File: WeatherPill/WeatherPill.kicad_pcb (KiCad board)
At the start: 2 copper layers, 319.5 x 201 mm, 61 parts, among them J1 Conn_01x02_Pin, J2 12402012E212A, J3 Conn_02x04_Odd_Even, J4 Conn_02x05_Odd_Even, J5 Conn_02x08_Odd_Even, Q1 PMOS, Q2 PMOS, SW2 SW_DPDT_x2, SW3 EVQ-P7A01P, SW4 EVQ-P7A01P, U1 USBLC6-2SC6, U2 STM32L052K8Tx, U3 sst25vf512a-33-4c-sae, U4 BU9796AMUV-E2, U5 BME280

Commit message: fred: avancements
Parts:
- removed the R1 at (26.6, 53.5)
- removed the R1 at (20.9, 67.5)
- removed the R15 at (108.5, 65.5)
- removed the R15 at (86.5, 94.5)
- removed R4: 0R, Capacitor_SMD:C_0603_1608Metric_Pad1.08x0.95mm_HandSolder
- added D1: LTST-C190GKT, green led:LEDM1608X80, F.Cu at (29.5, 70.0)
- added D2: LTST-C190GKT, green led:LEDM1608X80, F.Cu at (57.2, 65.5)
- added D3: LTST-C190GKT, green led:LEDM1608X80, F.Cu at (56.8, 86.0)
- added R1: 0R, Capacitor_SMD:C_0603_1608Metric_Pad1.08x0.95mm_HandSolder, F.Cu at (31.4, 47.5)
- added R15: 0R, Capacitor_SMD:C_0603_1608Metric_Pad1.08x0.95mm_HandSolder, F.Cu at (100.0, 45.0)
- added R29: 240R, Resistor_SMD:R_0603_1608Metric_Pad0.98x0.95mm_HandSolder, F.Cu at (31.0, 69.0)
- added R30: 240R, Resistor_SMD:R_0603_1608Metric_Pad0.98x0.95mm_HandSolder, F.Cu at (54.7, 66.0)
- added R31: 240R, Resistor_SMD:R_0603_1608Metric_Pad0.98x0.95mm_HandSolder, F.Cu at (54.3, 86.5)
- BT1: moved to B.Cu
- moved H1 63.8 mm to (107.0, 67.0)
- moved H2 63.8 mm to (107.5, 79.5)
- moved H3 63.8 mm to (89.5, 80.5)
- moved H4 63.8 mm to (103.5, 91.5)
- moved SW4 49.8 mm to (29.5, 88.7), turned to 0 degrees
- moved SW3 49.6 mm to (37.5, 88.7), turned to 0 degrees
- moved R21 48.4 mm to (95.1, 46.5), turned to 0 degrees
- moved R22 45.6 mm to (95.1, 49.0), turned to 0 degrees
- moved R28 45.0 mm to (89.0, 53.0), turned to 0 degrees
- moved R8 43.8 mm to (41.7, 86.2), turned to 0 degrees
- moved C6 42.6 mm to (29.5, 85.2), turned to 0 degrees
- moved C5 42.4 mm to (37.4, 84.7), turned to 0 degrees
- moved R13 42.1 mm to (24.9, 85.7), turned to 0 degrees
- moved R27 41.0 mm to (90.0, 56.0), turned to 0 degrees
- moved R26 36.7 mm to (90.5, 59.5), turned to 0 degrees
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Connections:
- U2 pad 2: Net-(U2-PC14) -> LED0
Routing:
- net GND: track 103.0 -> 0.00 mm, vias 22 -> 0
- net V_BUS_3V: track 73.5 -> 0.00 mm
- net V_BUS_ZONE_1: track 60.9 -> 0.00 mm, vias 2 -> 0
- net SDO_1: track 60.5 -> 0.00 mm
- net CONTROL_ZONE_2: track 51.8 -> 0.00 mm
- net SCK_1: track 50.8 -> 0.00 mm
- net SDI_1: track 46.0 -> 0.00 mm
- net Net-(J1-Pin_1): track 45.2 -> 0.00 mm, vias 2 -> 0
- net CONTROL_ZONE_1: track 41.6 -> 0.00 mm
- net CS_2: track 40.8 -> 0.00 mm
- net V_BUS_ZONE_2: track 35.1 -> 0.00 mm, vias 2 -> 0
- net SDI_SST25: track 33.2 -> 0.00 mm
- net CS_BME280: track 32.4 -> 0.00 mm
- net NRST: track 31.3 -> 0.00 mm, vias 2 -> 0
- net SCK_SST25: track 29.5 -> 0.00 mm
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- added copper zone on F.Cu, net GND
- added copper zone on In1.Cu, net GND
- added copper zone on In2.Cu, net GND
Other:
- board size 319.5 x 201 mm -> 96.8 x 58.8 mm
- copper layers 2 -> 4

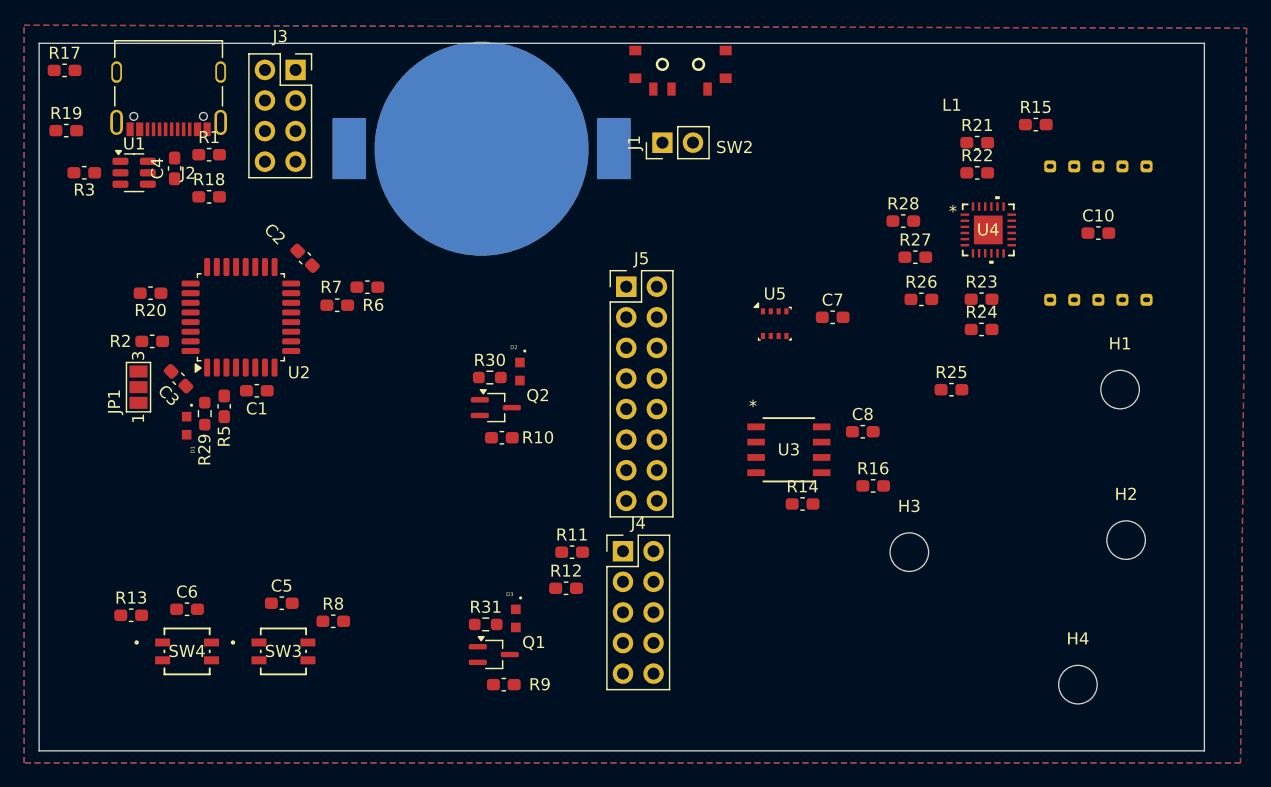
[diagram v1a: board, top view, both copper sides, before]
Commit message: V2 cooking
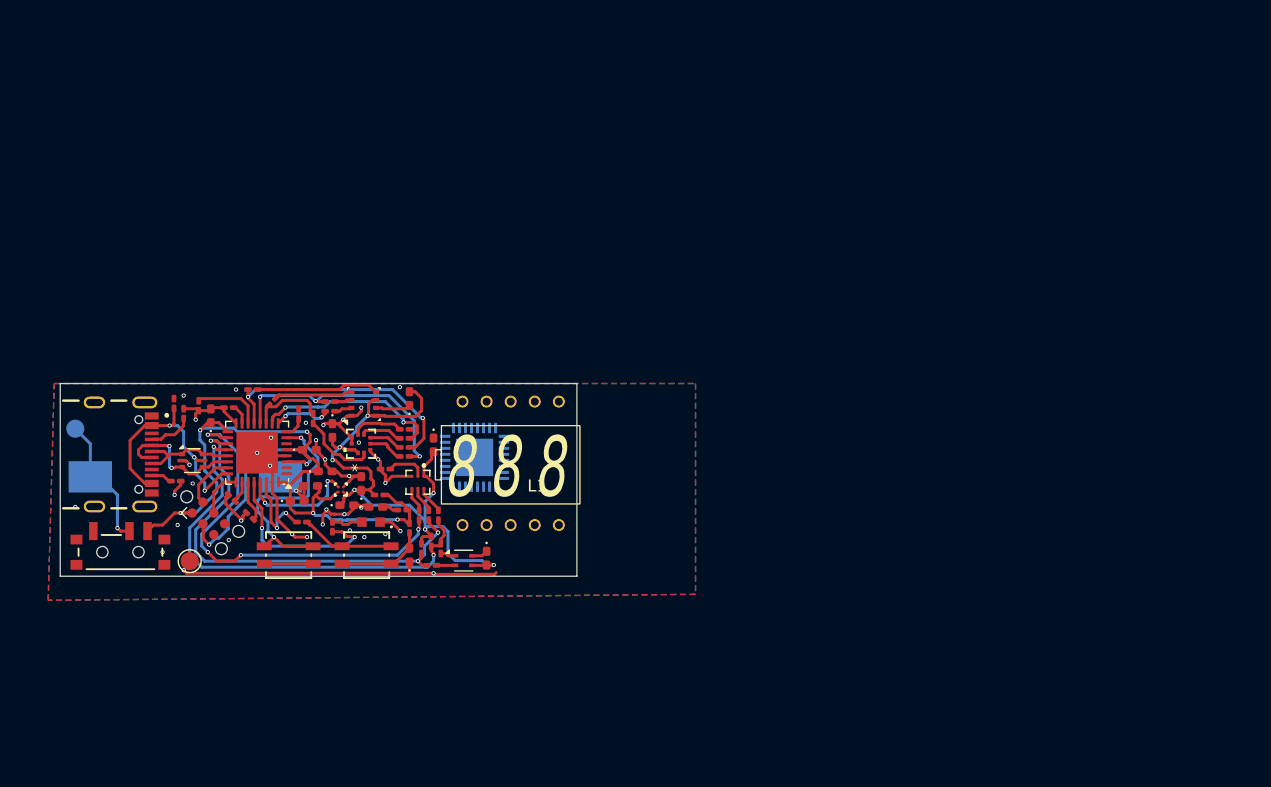
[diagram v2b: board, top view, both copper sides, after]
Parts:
- removed D2, D3: LTST-C190GKT, green led:LEDM1608X80
- removed H1, H2, H3, H4: MountingHole, MountingHole:MountingHole_3.2mm_M3_DIN965
- removed J3: Conn_02x04_Odd_Even, Connector_PinSocket_2.54mm:PinSocket_2x04_P2.54mm_Vertical
- removed J4: Conn_02x05_Odd_Even, Connector_PinHeader_2.54mm:PinHeader_2x05_P2.54mm_Vertical
- removed J5: Conn_02x08_Odd_Even, Connector_PinHeader_2.54mm:PinHeader_2x08_P2.54mm_Vertical
- removed JP1: SolderJumper_3_Open, Jumper:SolderJumper-3_P1.3mm_Open_Pad1.0x1.5mm_NumberLabels
- removed Q1, Q2: PMOS, Package_TO_SOT_SMD:SOT-323_SC-70_Handsoldering
- removed R21, R22, R23, R24, R25, R26, R27, R28: 0R, Capacitor_SMD:C_0603_1608Metric_Pad1.08x0.95mm_HandSolder
- removed SW2: SW_DPDT_x2, dpdt_switch:450404015514
- added C11: 1uf, LED_SMD:LED_0402_1005Metric_Pad0.77x0.64mm_HandSolder, F.Cu at (39.8, 75.0)
- added C12: 1uf, LED_SMD:LED_0402_1005Metric_Pad0.77x0.64mm_HandSolder, F.Cu at (44.0, 74.8)
- added C13: 100nF, LED_SMD:LED_0402_1005Metric_Pad0.77x0.64mm_HandSolder, F.Cu at (42.8, 76.6)
- added C9: 100nF, LED_SMD:LED_0402_1005Metric_Pad0.77x0.64mm_HandSolder, F.Cu at (41.6, 70.4)
- added R32: 0R, Resistor_SMD:R_0201_0603Metric_Pad0.64x0.40mm_HandSolder, F.Cu at (46.0, 73.6)
- added R33: 0R, Resistor_SMD:R_0201_0603Metric_Pad0.64x0.40mm_HandSolder, F.Cu at (48.8, 77.4)
- added R34: 0R, Resistor_SMD:R_0201_0603Metric_Pad0.64x0.40mm_HandSolder, F.Cu at (47.6, 71.8)
- added R35: 0R, Resistor_SMD:R_0201_0603Metric_Pad0.64x0.40mm_HandSolder, F.Cu at (40.0, 69.4)
- added R36: 0R, Resistor_SMD:R_0201_0603Metric_Pad0.64x0.40mm_HandSolder, F.Cu at (47.6, 72.5)
- added R37: 0R, Resistor_SMD:R_0201_0603Metric_Pad0.64x0.40mm_HandSolder, F.Cu at (47.6, 71.0)
- added R38: 0R, Resistor_SMD:R_0201_0603Metric_Pad0.64x0.40mm_HandSolder, F.Cu at (47.6, 70.3)
- added R4: 5.1k, Resistor_SMD:R_0201_0603Metric_Pad0.64x0.40mm_HandSolder, F.Cu at (29.2, 69.0)
- added SW1: CUS-12TB, batt_switch:CUS-12TB_NDC, F.Cu at (24.0, 80.5)
- added TP1: VBATT, TestPoint:TestPoint_Pad_D1.5mm, B.Cu at (20.2, 70.2)
- added TP2: GND, TestPoint:TestPoint_Pad_D1.5mm, F.Cu at (29.8, 81.2)
- added U6: HDC2010YPAR, HDC:BGA6C100X50P2X3_HDC2010YPAR, F.Cu at (48.7, 74.7)
- added U7: BMP581, bmp581:QFN10_BMP581_BOS-M, F.Cu at (44.0, 71.5)
- added U8: STM32L072KZUx, Package_DFN_QFN:QFN-32-1EP_5x5mm_P0.5mm_EP3.45x3.45mm, F.Cu at (35.4, 72.2)
- BT1: value BK-912-TR -> 1056; footprint bk-912-tr:MPD_BK-912-TR -> batt12mm:BAT_1056
- C1, C10, C2, C3, C4, C5, C6, C7: footprint Capacitor_SMD:C_0603_1608Metric_Pad1.08x0.95mm_HandSolder -> LED_SMD:LED_0402_1005Metric_Pad0.77x0.64mm_HandSolder
- C8: value 0.1uF -> 100nF; footprint Capacitor_SMD:C_0603_1608Metric_Pad1.08x0.95mm_HandSolder -> LED_SMD:LED_0402_1005Metric_Pad0.77x0.64mm_HandSolder
- J1: value Conn_01x02_Pin -> Conn_ARM_SWD_TagConnect_TC2030-NL; footprint Connector_PinHeader_2.54mm:PinHeader_1x02_P2.54mm_Vertical -> Connector:Tag-Connect_TC2030-IDC-NL_2x03_P1.27mm_Vertical
- J2: value 12402012E212A -> USB4105-GF-A; footprint USB12402012E212A:AMPHENOL_12402012E212A -> usb conn atomic:GCT_USB4105-GF-A
- L1: footprint Library:lcd_ebay -> led7segment:INND-SS30
- R1, R11, R12, R13, R14, R15, R16, R17, R18, R19, R20, R5, R6, R7, R8: footprint Capacitor_SMD:C_0603_1608Metric_Pad1.08x0.95mm_HandSolder -> Resistor_SMD:R_0201_0603Metric_Pad0.64x0.40mm_HandSolder
- R10, R9: value 1M -> 0R; footprint Capacitor_SMD:C_0603_1608Metric_Pad1.08x0.95mm_HandSolder -> Resistor_SMD:R_0201_0603Metric_Pad0.64x0.40mm_HandSolder
- R2: value 1M -> 1K; footprint Capacitor_SMD:C_0603_1608Metric_Pad1.08x0.95mm_HandSolder -> Resistor_SMD:R_0201_0603Metric_Pad0.64x0.40mm_HandSolder
- R29: value 240R -> 470R; footprint Resistor_SMD:R_0603_1608Metric_Pad0.98x0.95mm_HandSolder -> Resistor_SMD:R_0201_0603Metric_Pad0.64x0.40mm_HandSolder
- R3: value 0R -> 5.1k; footprint Capacitor_SMD:C_0603_1608Metric_Pad1.08x0.95mm_HandSolder -> Resistor_SMD:R_0201_0603Metric_Pad0.64x0.40mm_HandSolder
- R30, R31: value 240R -> 0R; footprint Resistor_SMD:R_0603_1608Metric_Pad0.98x0.95mm_HandSolder -> Resistor_SMD:R_0201_0603Metric_Pad0.64x0.40mm_HandSolder
- U1: value USBLC6-2SC6 -> USBLC6-2P6; footprint Package_TO_SOT_SMD:SOT-23-6 -> Package_TO_SOT_SMD:SOT-666
- U2: value STM32L052K8Tx -> ~; footprint Package_QFP:LQFP-32_7x7mm_P0.8mm -> Package_DFN_QFN:HVQFN-32-1EP_5x5mm_P0.5mm_EP3.1x3.1mm; moved to B.Cu
- U3: value sst25vf512a-33-4c-sae -> SHT4x; footprint sst25vf5:SOIC8_SA_SST_MCH -> Sensor_Humidity:Sensirion_DFN-4_1.5x1.5mm_P0.8mm_SHT4x_NoCentralPad
- U4: value BU9796AMUV-E2 -> TPS22916CYFPR; footprint lcd driver:VQFN024V4040_ROM -> loadswitch:YFP0004ABAB
- moved C10 67.2 mm to (41.0, 73.8)
- moved R15 62.6 mm to (45.5, 75.8), turned to 180 degrees
- moved U4 57.9 mm to (42.3, 75.3), turned to 180 degrees
- moved R16 50.4 mm to (36.6, 68.0), turned to -135 degrees
- moved J1 48.9 mm to (31.3, 77.7), turned to -45 degrees
- moved L1 46.9 mm to (64.2, 79.5)
- moved R14 46.6 mm to (35.0, 67.0), turned to 180 degrees
- moved C4 41.5 mm to (54.4, 81.0), turned to -90 degrees
- moved R1 38.8 mm to (49.8, 81.6), turned to 180 degrees
- moved BT1 36.5 mm to (29.7, 74.2)
- moved C7 35.8 mm to (48.0, 67.8), turned to 90 degrees
- moved C8 35.7 mm to (50.0, 71.6), turned to -90 degrees
- moved R17 35.2 mm to (41.4, 68.0), turned to 180 degrees
- moved U5 34.8 mm to (44.2, 68.2), turned to 90 degrees
- moved J2 32.3 mm to (21.8, 72.4), turned to -90 degrees
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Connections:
- C10 pad 1: V_BUS_DISPLAY -> V_BUS_3V
- C4 pad 1: USB_D+ -> GND
- C4 pad 2: USB_D- -> V_BUS_ZONE_1
- J1 pad 1: Net-(J1-Pin_1) -> V_BUS_3V
- J1 pad 2: GND -> SWDIO
- J2 pad A1_B12: Net-(U1-GND) -> GND
- J2 pad A4_B9: Net-(U1-VBUS) -> V_USB
- J2 pad A5: Net-(J2-CC1-PadA5) -> Net-(J2-CC1)
- J2 pad A6: Net-(J2-D+-PadA6) -> USB_D+
- J2 pad A7: Net-(J2-D--PadA7) -> USB_D-
- J2 pad A8: Net-(J2-SBU1) -> unconnected-(J2-SBU1-PadA8)
- J2 pad B1_A12: Net-(U1-GND) -> GND
- J2 pad B4_A9: Net-(U1-VBUS) -> V_USB
- J2 pad B5: Net-(J2-CC1-PadB5) -> Net-(J2-CC2)
- J2 pad B6: Net-(J2-D+-PadA6) -> USB_D+
- J2 pad B7: Net-(J2-D--PadA7) -> USB_D-
- J2 pad B8: Net-(J2-SBU2) -> unconnected-(J2-SBU2-PadB8)
- J2 pad SH1: (no net) -> GND
- J2 pad SH2: (no net) -> GND
- J2 pad SH3: (no net) -> GND
- J2 pad SH4: (no net) -> GND
- L1 pad 1: Net-(U4-SEG0) -> unconnected-(L1-Pad1)
- L1 pad 10: Net-(U4-COM0) -> unconnected-(L1-Pad10)
- L1 pad 2: Net-(U4-SEG1) -> unconnected-(L1-Pad2)
- L1 pad 3: Net-(U4-SEG2) -> unconnected-(L1-Pad3)
- L1 pad 4: Net-(U4-SEG3) -> unconnected-(L1-Pad4)
- L1 pad 5: Net-(U4-SEG4) -> unconnected-(L1-Pad5)
- L1 pad 6: Net-(U4-SEG8) -> unconnected-(L1-Pad6)
- L1 pad 7: Net-(U4-COM2) -> unconnected-(L1-Pad7)
- L1 pad 8: Net-(U4-COM2) -> unconnected-(L1-Pad8)
- L1 pad 9: Net-(U4-COM0) -> unconnected-(L1-Pad9)
- R1 pad 1: Net-(J2-CC1-PadA5) -> Net-(U3-SCL)
- R1 pad 2: GND -> SCL_1
- R10 pad 1: V_BUS_3V -> Net-(U3-SDA)
- R10 pad 2: CONTROL_ZONE_1 -> SDA_1
- R11 pad 2: V_BUS_ZONE_2 -> V_BUS_ZONE_1
- R12 pad 2: V_BUS_ZONE_2 -> V_BUS_ZONE_1
- R14 pad 1: V_BUS_ZONE_1 -> Net-(U5-SDO)
- R14 pad 2: Net-(U3-*WP) -> SDO_1
- R15 pad 1: Net-(U4-OSCIN) -> V_BUS_3V
- R15 pad 2: GND -> V_BUS_ZONE_1
- R16 pad 1: Net-(U3-*HOLD) -> Net-(U5-SCK)
- R16 pad 2: GND -> SCK_1
- R17 pad 1: Net-(J2-CC1-PadB5) -> Net-(U5-SDI)
- R17 pad 2: GND -> SDI_1
- R18 pad 1: GND -> Net-(U5-CSB)
- R18 pad 2: Net-(J2-SBU2) -> CS_1
- R19 pad 1: Net-(J2-SBU1) -> V_USB
- R19 pad 2: GND -> unconnected-(R19-Pad2)
- R2 pad 1: BOOT -> BTN_2
- R20 pad 1: Net-(U2-PB3) -> Net-(U8-PB4)
- R29 pad 1: LED0 -> Net-(U8-PB6)
- R3 pad 1: Net-(U1-GND) -> GND
- R3 pad 2: GND -> Net-(J2-CC2)
- R30 pad 1: V_BUS_ZONE_1 -> Net-(U6-SCL)
- R30 pad 2: Net-(D2-PadA) -> SCL_1
- R31 pad 1: V_BUS_ZONE_2 -> Net-(U6-SDA)
- R31 pad 2: Net-(D3-PadA) -> SDA_1
- R5 pad 1: Net-(U2-PC15) -> unconnected-(R5-Pad1)
- R5 pad 2: GND -> Net-(U8-PA2)
- R6 pad 1: Net-(U2-PB0) -> Net-(U8-PB0)
- R7 pad 1: Net-(U2-PB1) -> Net-(U8-PB1)
- R9 pad 1: V_BUS_3V -> Net-(U8-PB5)
- R9 pad 2: CONTROL_ZONE_2 -> GND
- SW4 pad 2: GND -> Net-(C6-Pad2)
- U1 pad 1: Net-(J2-D--PadA7) -> USB_D+
- U1 pad 2: Net-(U1-GND) -> GND
- U1 pad 3: Net-(J2-D+-PadA6) -> USB_D-
- U1 pad 4: USB_D+ -> USB_D-
- U1 pad 5: Net-(U1-VBUS) -> V_USB
- U1 pad 6: USB_D- -> USB_D+
- U2 pad 1: V_BUS_3V -> unconnected-(U2-COM3-Pad1)
- U2 pad 10: CS_2 -> unconnected-(U2-PORE-Pad10)
- U2 pad 11: SCK_1 -> unconnected-(U2-A1-Pad11)
- U2 pad 12: SDI_1 -> unconnected-(U2-SEG0-Pad12)
- U2 pad 13: SDO_1 -> unconnected-(U2-SEG1-Pad13)
- U2 pad 14: Net-(U2-PB0) -> unconnected-(U2-SEG2-Pad14)
- U2 pad 15: Net-(U2-PB1) -> unconnected-(U2-SEG3-Pad15)
- U2 pad 16: GND -> unconnected-(U2-SEG4-Pad16)
- U2 pad 17: V_BUS_3V -> unconnected-(U2-SEG5-Pad17)
- U2 pad 18: BTN_2 -> unconnected-(U2-SEG6-Pad18)
- U2 pad 19: BTN_1 -> unconnected-(U2-SEG7-Pad19)
- U2 pad 2: LED0 -> unconnected-(U2-VLCD-Pad2)
- U2 pad 20: GND -> unconnected-(U2-SEG8-Pad20)
- U2 pad 21: USB_D- -> unconnected-(U2-SEG9-Pad21)
- U2 pad 22: USB_D+ -> unconnected-(U2-SEG10-Pad22)
- U2 pad 23: SWDIO -> unconnected-(U2-SEG11-Pad23)
- U2 pad 24: SWCLK -> unconnected-(U2-SEG12-Pad24)
- U2 pad 25: GND -> unconnected-(U2-SEG13-Pad25)
- U2 pad 26: Net-(U2-PB3) -> unconnected-(U2-SEG14-Pad26)
- U2 pad 27: CONTROL_ZONE_2 -> unconnected-(U2-SEG15-Pad27)
- U2 pad 28: CONTROL_ZONE_1 -> unconnected-(U2-SEG16-Pad28)
- U2 pad 29: SCL_1 -> unconnected-(U2-SEG17-Pad29)
- U2 pad 3: Net-(U2-PC15) -> unconnected-(U2-VDD-Pad3)
- U2 pad 30: SDA_1 -> unconnected-(U2-COM0-Pad30)
- U2 pad 31: BOOT -> unconnected-(U2-COM1-Pad31)
- U2 pad 32: GND -> unconnected-(U2-COM2-Pad32)
- U2 pad 4: NRST -> unconnected-(U2-VSS-Pad4)
- U2 pad 5: V_BUS_3V -> unconnected-(U2-_RST-Pad5)
- U2 pad 6: GND -> unconnected-(U2-A0-Pad6)
- U2 pad 7: GND -> unconnected-(U2-CLK-Pad7)
- U2 pad 8: GND -> unconnected-(U2-SCL-Pad8)
- U2 pad 9: CS_1 -> unconnected-(U2-SDA-Pad9)
- U3 pad 1: CS_SST25 -> Net-(U3-SDA)
- U3 pad 2: SDO_SST25 -> Net-(U3-SCL)
- U3 pad 3: Net-(U3-*WP) -> V_BUS_ZONE_1
- U5 pad 2: CS_BME280 -> Net-(U5-CSB)
- U5 pad 3: SDI_BME280 -> Net-(U5-SDI)
- U5 pad 4: SCK_BME280 -> Net-(U5-SCK)
- U5 pad 5: SDO_BME280 -> Net-(U5-SDO)
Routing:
- net GND: track 0.00 -> 86.9 mm, vias 0 -> 38
- net V_BUS_3V: track 0.00 -> 56.0 mm, vias 0 -> 5
- net V_BUS_ZONE_1: track 0.00 -> 54.4 mm, vias 0 -> 7
- net SCL_1: track 0.00 -> 37.7 mm, vias 0 -> 3
- net SDA_1: track 0.00 -> 37.0 mm, vias 0 -> 2
- net HDC_DRDY: track 0.00 -> 34.5 mm, vias 0 -> 4
- net SDO_1: track 0.00 -> 22.1 mm, vias 0 -> 2
- net SDI_1: track 0.00 -> 21.1 mm, vias 0 -> 3
- net V_USB: track 0.00 -> 20.4 mm, vias 0 -> 3
- net BTN_1: track 0.00 -> 19.6 mm, vias 0 -> 2
- net NRST: track 0.00 -> 19.5 mm, vias 0 -> 2
- net Net-(U8-PB6): track 0.00 -> 15.3 mm, vias 0 -> 2
- net CS_2: track 0.00 -> 15.1 mm, vias 0 -> 2
- net USB_D-: track 0.00 -> 11.6 mm, vias 0 -> 2
- net Net-(BT1-PadP): track 0.00 -> 10.5 mm, vias 0 -> 1
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- removed copper zone on In1.Cu, net GND
- removed copper zone on In2.Cu, net GND
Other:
- board size 96.8 x 58.8 mm -> 42.9 x 16 mm
- copper layers 4 -> 2
